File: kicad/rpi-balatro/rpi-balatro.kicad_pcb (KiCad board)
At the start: 2 copper layers, 51 parts, among them J1 Raspberry_Pi_4, U10 SM420561N, U11 SM420561N, U12 SM420561N, U13 SM420561N, U14 SM420561N, U15 SM420561N, U16 SM420561N, U17 SM420561N, U18 SM420561N, U19 SM420561N, U2 MAX7221xNG, U20 SM420561N, U21 SM420561N, U22 SM420561N, U23 SM420561N, U24 SM420561N, U25 SM420561N, U26 SM420561N, U27 SM420561N, U28 SM420561N, U29 SM420561N, U3 MAX7221xNG, U30 SM420561N, U31 SM420561N, U32 SM420561N, U33 SM420561N, U4 MAX7221xNG, U42 SM420561N, U43 SM420561N, U44 SM420561N, U45 SM420561N, U46 SM420561N, U47 SM420561N, U48 SM420561N, U49 SM420561N, U50 SM420561N, U51 SM420561N, U52 SM420561N, U53 SM420561N, U54 SM420561N, U55 SM420561N, U56 SM420561N, U57 SM420561N, U6 MAX7221xNG, U8 MAX7221xNG

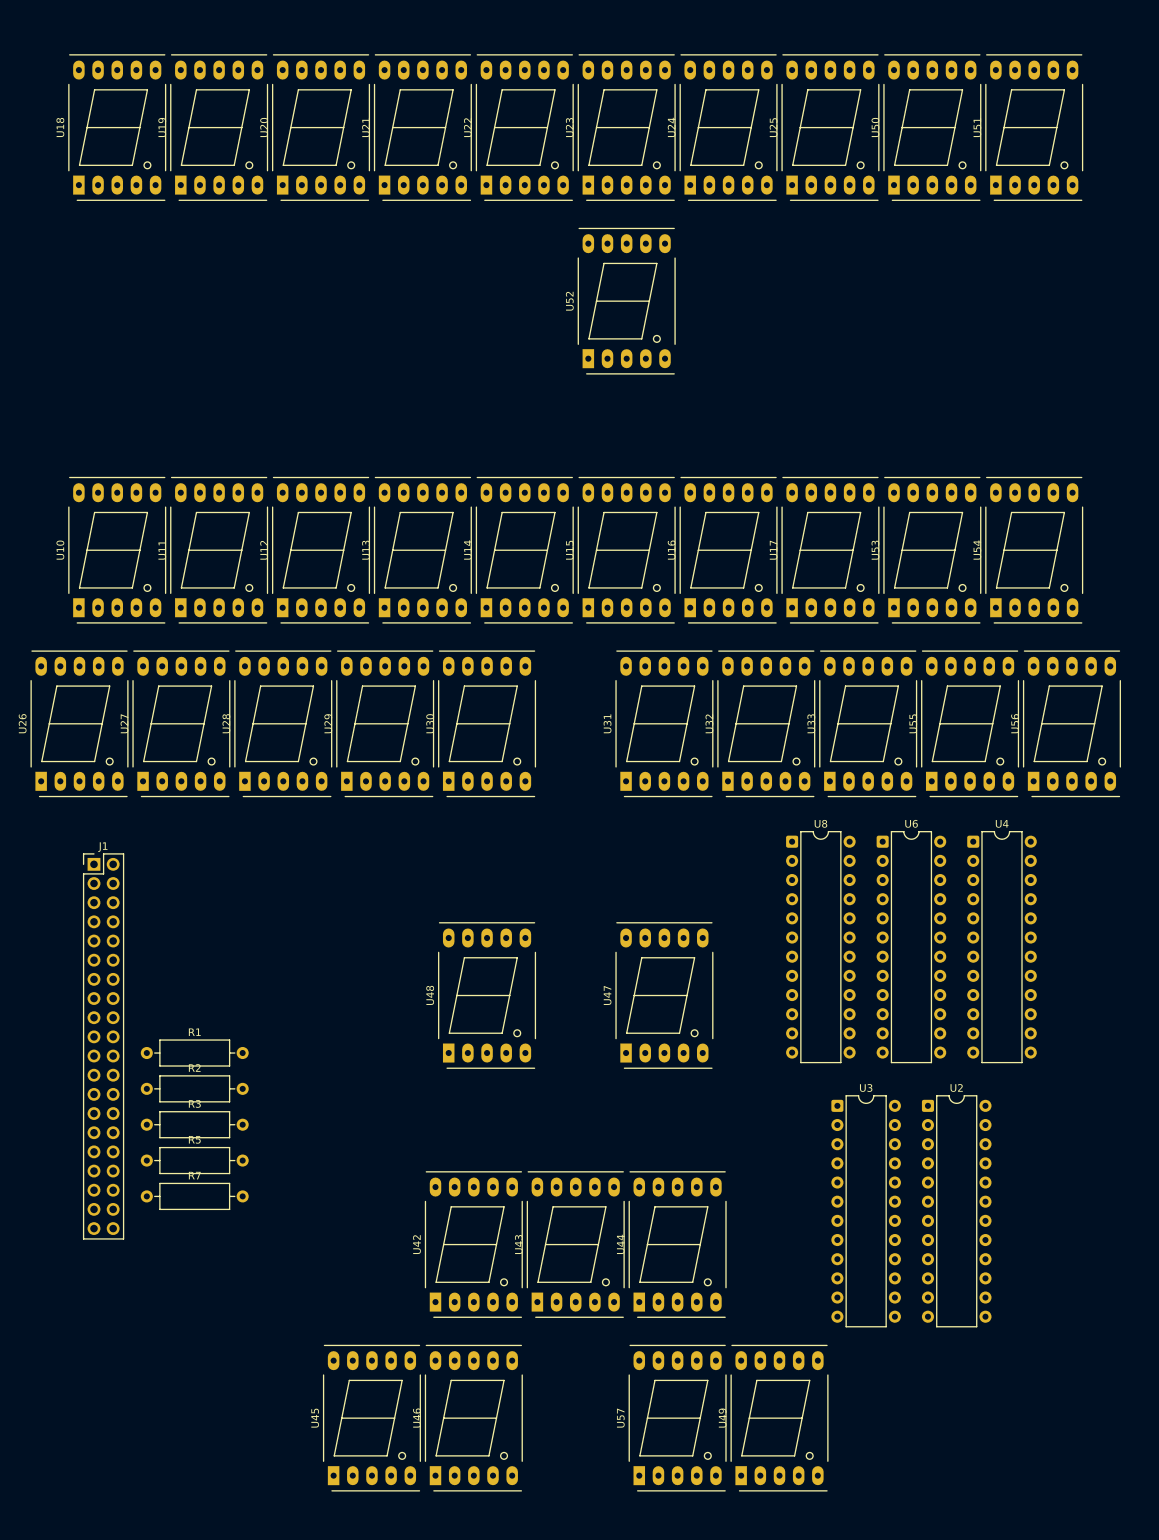
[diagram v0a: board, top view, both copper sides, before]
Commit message: addicted to pla
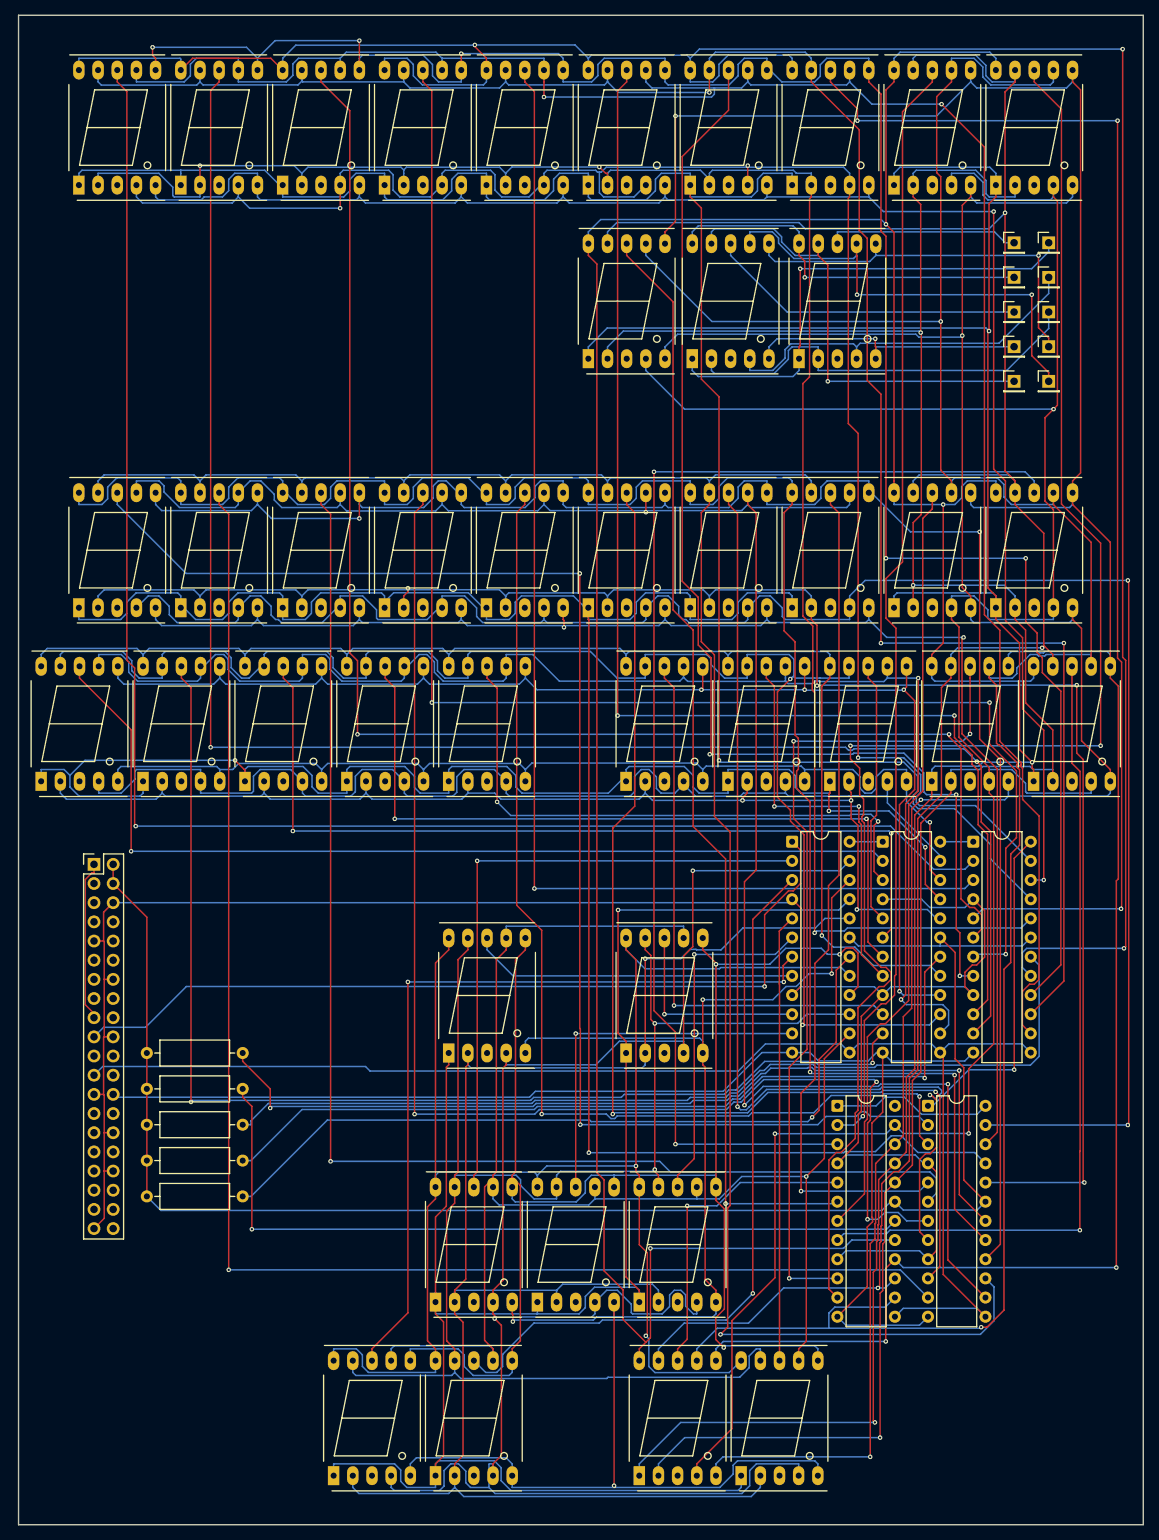
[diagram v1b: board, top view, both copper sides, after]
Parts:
- added J10: Conn_01x01_Socket, Connector_PinHeader_2.54mm:PinHeader_1x01_P2.54mm_Vertical, F.Cu at (151.5, 71.4)
- added J11: Conn_01x01_Socket, Connector_PinHeader_2.54mm:PinHeader_1x01_P2.54mm_Vertical, F.Cu at (151.5, 76.0)
- added J2: Conn_01x01_Socket, Connector_PinHeader_2.54mm:PinHeader_1x01_P2.54mm_Vertical, F.Cu at (146.9, 57.6)
- added J3: Conn_01x01_Socket, Connector_PinHeader_2.54mm:PinHeader_1x01_P2.54mm_Vertical, F.Cu at (146.9, 62.2)
- added J4: Conn_01x01_Socket, Connector_PinHeader_2.54mm:PinHeader_1x01_P2.54mm_Vertical, F.Cu at (146.9, 66.8)
- added J5: Conn_01x01_Socket, Connector_PinHeader_2.54mm:PinHeader_1x01_P2.54mm_Vertical, F.Cu at (146.9, 71.4)
- added J6: Conn_01x01_Socket, Connector_PinHeader_2.54mm:PinHeader_1x01_P2.54mm_Vertical, F.Cu at (146.9, 76.0)
- added J7: Conn_01x01_Socket, Connector_PinHeader_2.54mm:PinHeader_1x01_P2.54mm_Vertical, F.Cu at (151.5, 57.6)
- added J8: Conn_01x01_Socket, Connector_PinHeader_2.54mm:PinHeader_1x01_P2.54mm_Vertical, F.Cu at (151.5, 62.2)
- added J9: Conn_01x01_Socket, Connector_PinHeader_2.54mm:PinHeader_1x01_P2.54mm_Vertical, F.Cu at (151.5, 66.8)
- added U58: SM420561N, Display_7Segment:7SegmentLED_LTS6760_LTS6780, F.Cu at (104.3, 73.0)
- added U59: SM420561N, Display_7Segment:7SegmentLED_LTS6760_LTS6780, F.Cu at (118.4, 73.0)
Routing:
- net /digit_max_6/SEG_G: track 0.00 -> 371.0 mm, vias 0 -> 3
- net /digit_max_6/SEG_B: track 0.00 -> 337.7 mm, vias 0 -> 3
- net /digit_max_2/SEG_G: track 0.00 -> 328.6 mm, vias 0 -> 3
- net /digit_max_6/SEG_A: track 0.00 -> 327.7 mm, vias 0 -> 2
- net /digit_max_6/SEG_C: track 0.00 -> 321.0 mm, vias 0 -> 3
- net /digit_max_6/SEG_F: track 0.00 -> 312.4 mm, vias 0 -> 3
- net /digit_max_6/SEG_E: track 0.00 -> 310.6 mm, vias 0 -> 3
- net /digit_max_6/SEG_D: track 0.00 -> 301.1 mm, vias 0 -> 3
- net /digit_max_6/SEG_DP: track 0.00 -> 299.4 mm, vias 0 -> 3
- net /digit_max_2/SEG_B: track 0.00 -> 275.9 mm, vias 0 -> 5
- net Net-(J1-GND-Pad14): track 0.00 -> 273.7 mm
- net /digit_max_2/SEG_A: track 0.00 -> 272.0 mm, vias 0 -> 2
- net /digit_max_1/SEG_F: track 0.00 -> 268.2 mm, vias 0 -> 1
- net /digit_max_2/SEG_F: track 0.00 -> 267.9 mm, vias 0 -> 3
- net /digit_max_2/SEG_E: track 0.00 -> 257.6 mm, vias 0 -> 1
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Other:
- board outline added: 149 x 200 mm
